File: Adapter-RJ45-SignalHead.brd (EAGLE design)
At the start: 30.5 x 38.1 mm, 4 parts, among them CON1 CONNECTOR-GROVE-4P-2.0-347013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, CON2 CONNECTOR-GROVE-4P-2.0-347013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

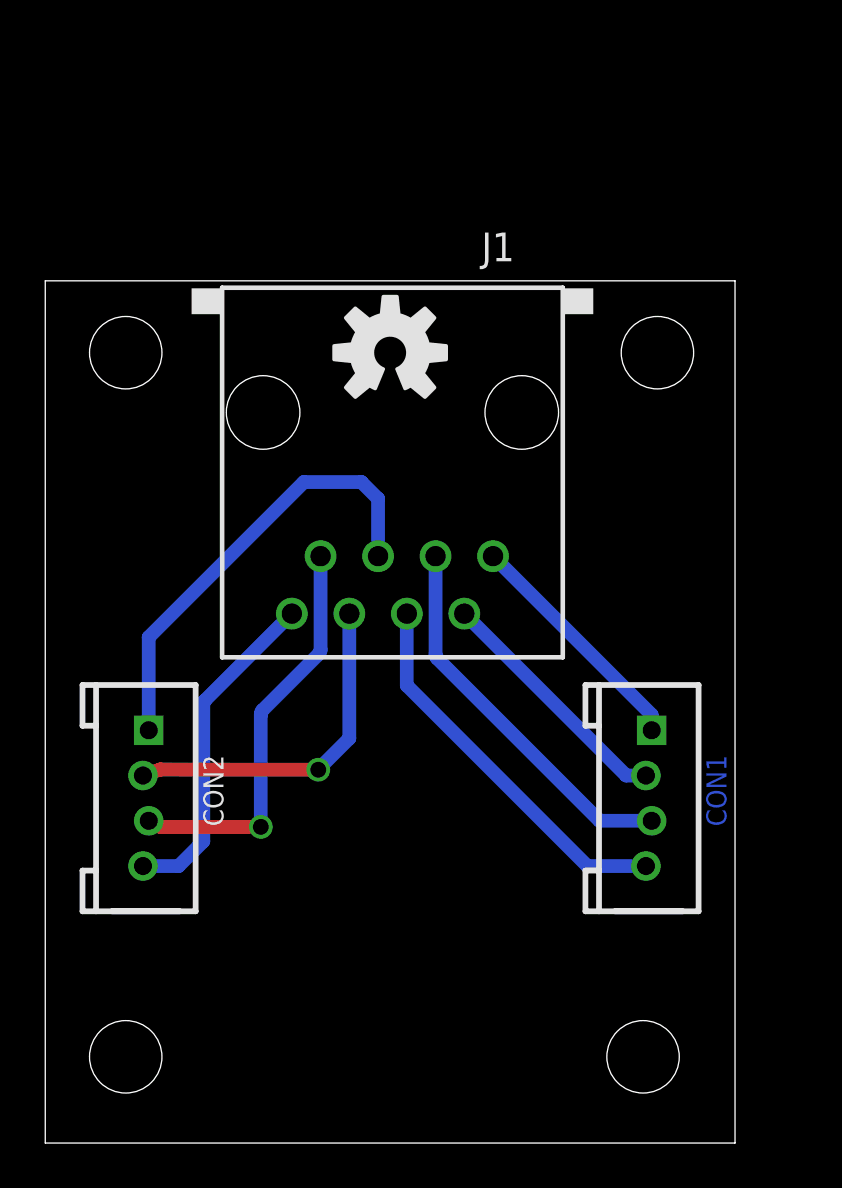
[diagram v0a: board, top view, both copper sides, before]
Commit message: V3.2 - added CUT-R
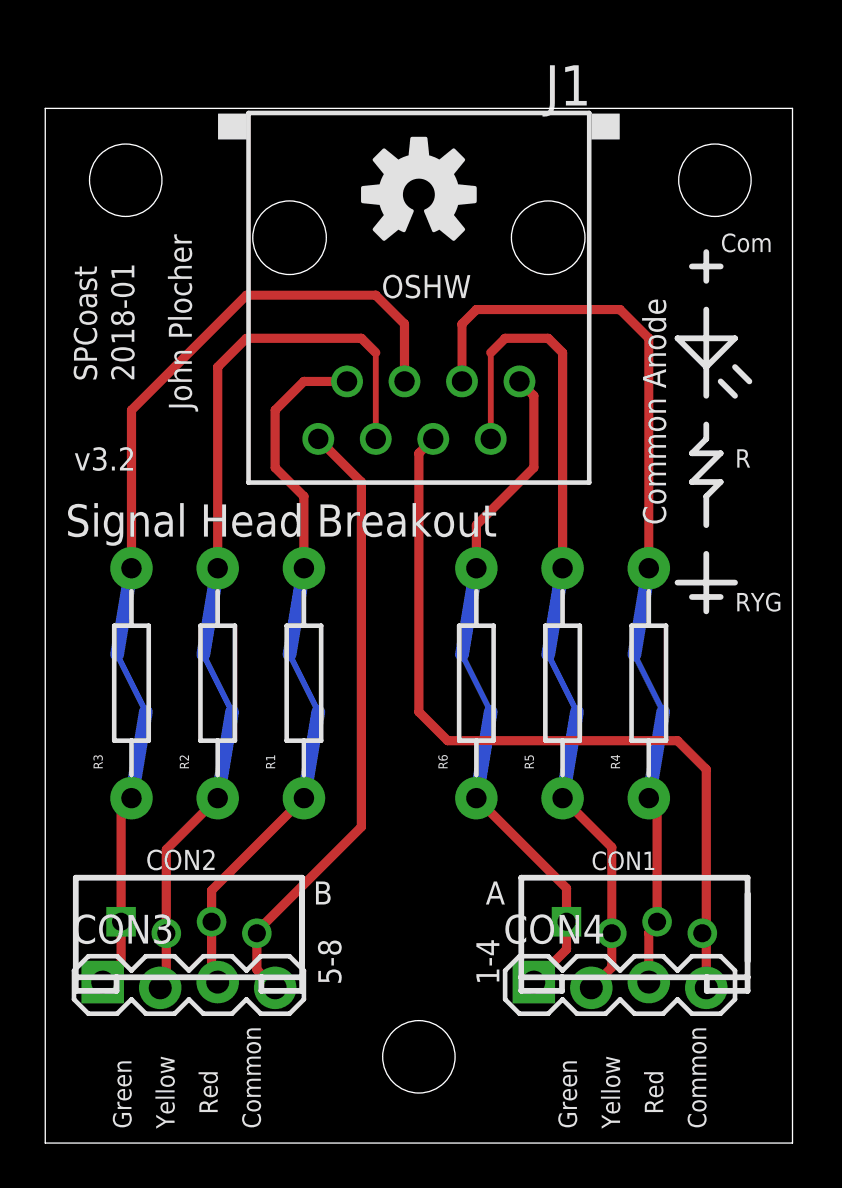
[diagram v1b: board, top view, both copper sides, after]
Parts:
- added CON3, CON4: (no value), SPCoast:1X04_LOCK
- added R1, R2, R3, R4, R5, R6: (no value), SPCoast:CUT-R
- CON1, CON2: value CONNECTOR-GROVE-4P-2.0-3470130P1 -> (none)
- moved J1 7.81 mm to (16.5, 40.0)
- moved U$1 7.10 mm to (16.5, 41.9)
- moved CON2 6.02 mm to (6.35, 9.53), turned to 0 degrees
- moved CON1 5.75 mm to (26.0, 9.53), turned to 0 degrees
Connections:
- removed net L5: CON2.1, J1.5
- removed net L6: CON2.2, J1.6
- removed net L7: CON2.3, J1.7
- removed net L8: CON2.4, J1.8
- removed net N$1: CON1.1, J1.1
- removed net N$2: CON1.2, J1.2
- removed net N$3: CON1.3, J1.3
- removed net N$4: CON1.4, J1.4
- new net A-COMMON: CON1.4, CON4.4, J1.4
- new net AG: J1.1, R6.P1
- new net AGR: CON1.1, CON4.1, R6.P2
- new net AR: J1.3, R4.P1
- new net ARR: CON1.3, CON4.3, R4.P2
- new net AY: J1.2, R5.P1
- new net AYR: CON1.2, CON4.2, R5.P2
- new net B-COMMON: CON2.4, CON3.4, J1.8
- new net BG: J1.5, R3.P1
- new net BGR: CON2.1, CON3.1, R3.P2
- new net BR: J1.7, R1.P1
- new net BRR: CON2.3, CON3.3, R1.P2
- new net BY: J1.6, R2.P1
- new net BYR: CON2.2, CON3.2, R2.P2
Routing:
- net A-COMMON: track 0.00 -> 35.9 mm
- net B-COMMON: track 0.00 -> 27.3 mm
- net BG: track 0.00 -> 24.2 mm
- net AR: track 0.00 -> 21.7 mm
- net BY: track 0.00 -> 20.5 mm
- net L5: track 19.9 -> 0.00 mm
- net L7: track 18.0 -> 0.00 mm, vias 1 -> 0
- net N$4: track 17.0 -> 0.00 mm
- net AY: track 0.00 -> 17.0 mm
- net N$3: track 17.0 -> 0.00 mm
- net L6: track 15.3 -> 0.00 mm, vias 1 -> 0
- net L8: track 14.8 -> 0.00 mm
- net BR: track 0.00 -> 11.2 mm
- net N$2: track 11.0 -> 0.00 mm
- net N$1: track 10.6 -> 0.00 mm
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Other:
- board size 30.5 x 38.1 mm -> 33 x 45.7 mm
- board text added: "CON1"
- board text added: "CON2"
- board text added: "CON3"
- board text added: "CON4"
- board text added: "Com"
- board text added: "Common"
- board text added: "Common Anode"
- board text added: "Cut traces is using resistors"
- board text added: "J1"
- board text added: "OSHW"
- board text added: "R"
- board text added: "R1"
- board text added: "R2"
- board text added: "R3"
- board text added: "R4"
- board text added: "R5"
- board text added: "R6"
- board text added: "RYG"
- board text added: "Signal Head Breakout"
- board text added: "v3.2"
- board text added: "www. SPCoast .com"
- board text removed: "+ Common +"
- board text removed: ".com"
- board text removed: "Go Bears!"
- board text removed: "SP Coast"
- board text removed: "v3.1"
- board text removed: "www."
